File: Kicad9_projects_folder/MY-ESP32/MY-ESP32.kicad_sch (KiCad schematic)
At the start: 67 parts, among them J1 SM04B-SRSS-TB, J2 SM04B-SRSS-TB, Q1 2N3904S-RTK/PS, Q2 2N3904S-RTK/PS, Q5 PMOSFET-DMP1045U-7, SW3 SPDT, U1 USBLC6-2SC6, U3 CP2102N-Axx-xQFN28, U4 DFR0819, U7 USB4110GFA

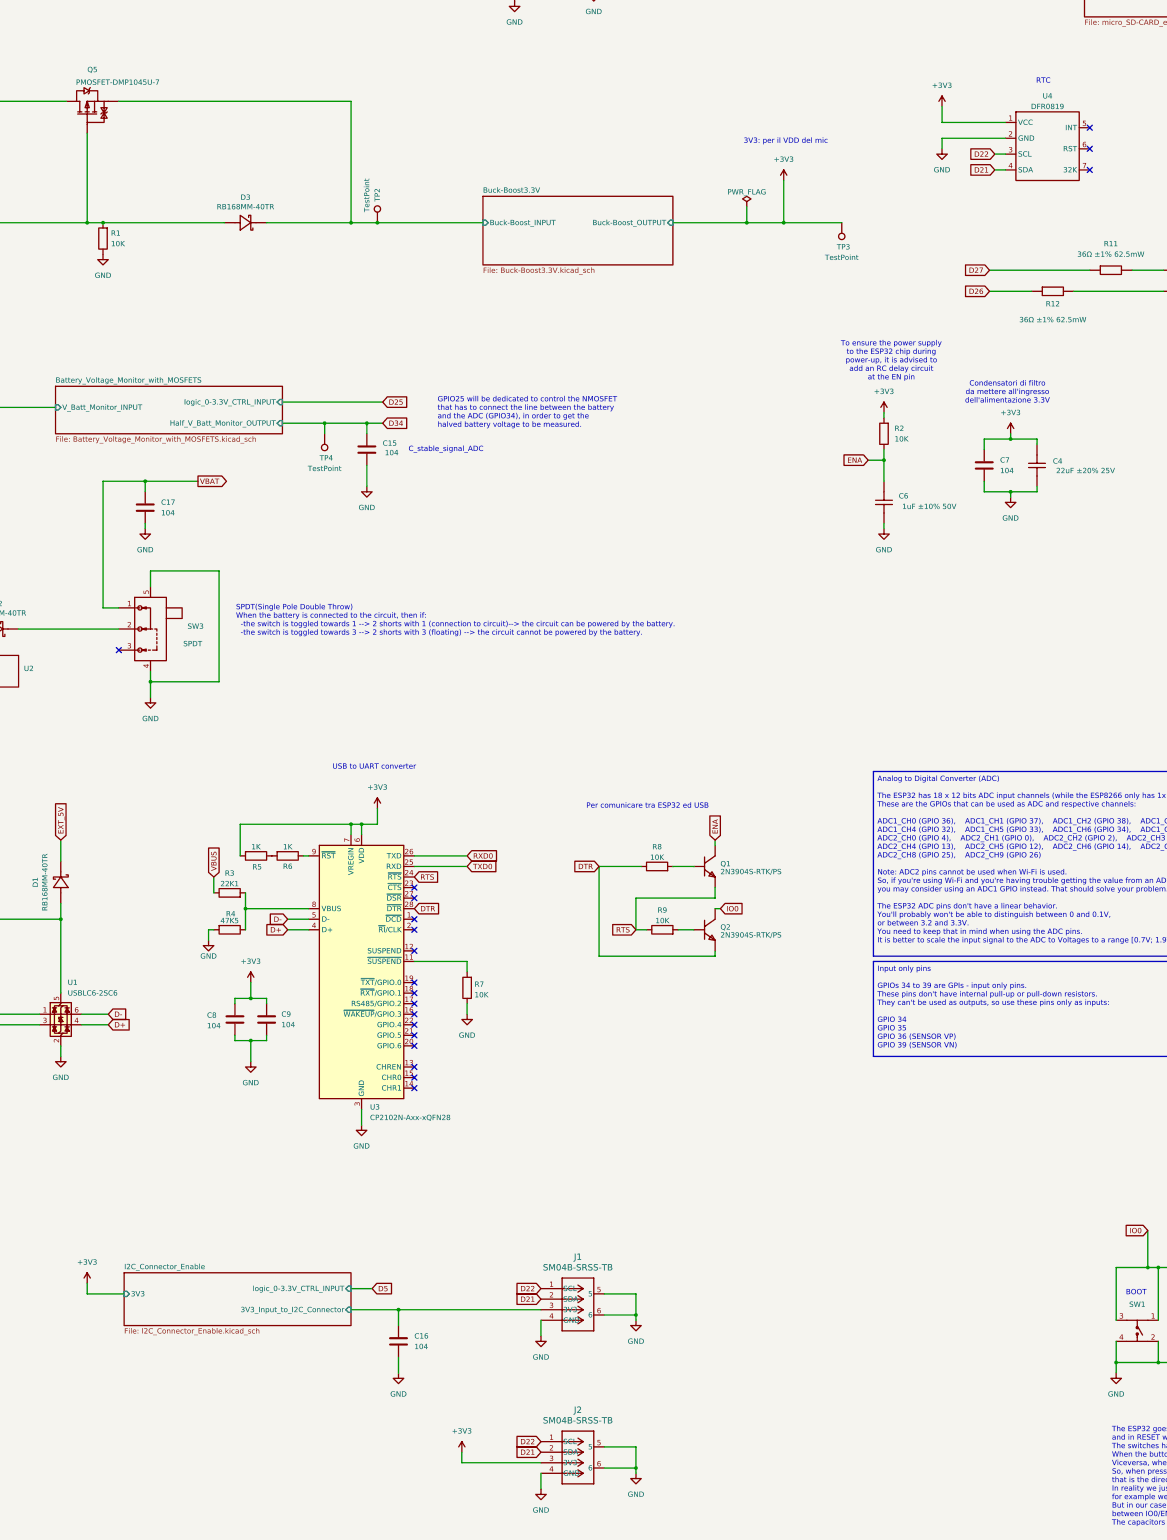
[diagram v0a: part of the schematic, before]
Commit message: Fourth commit
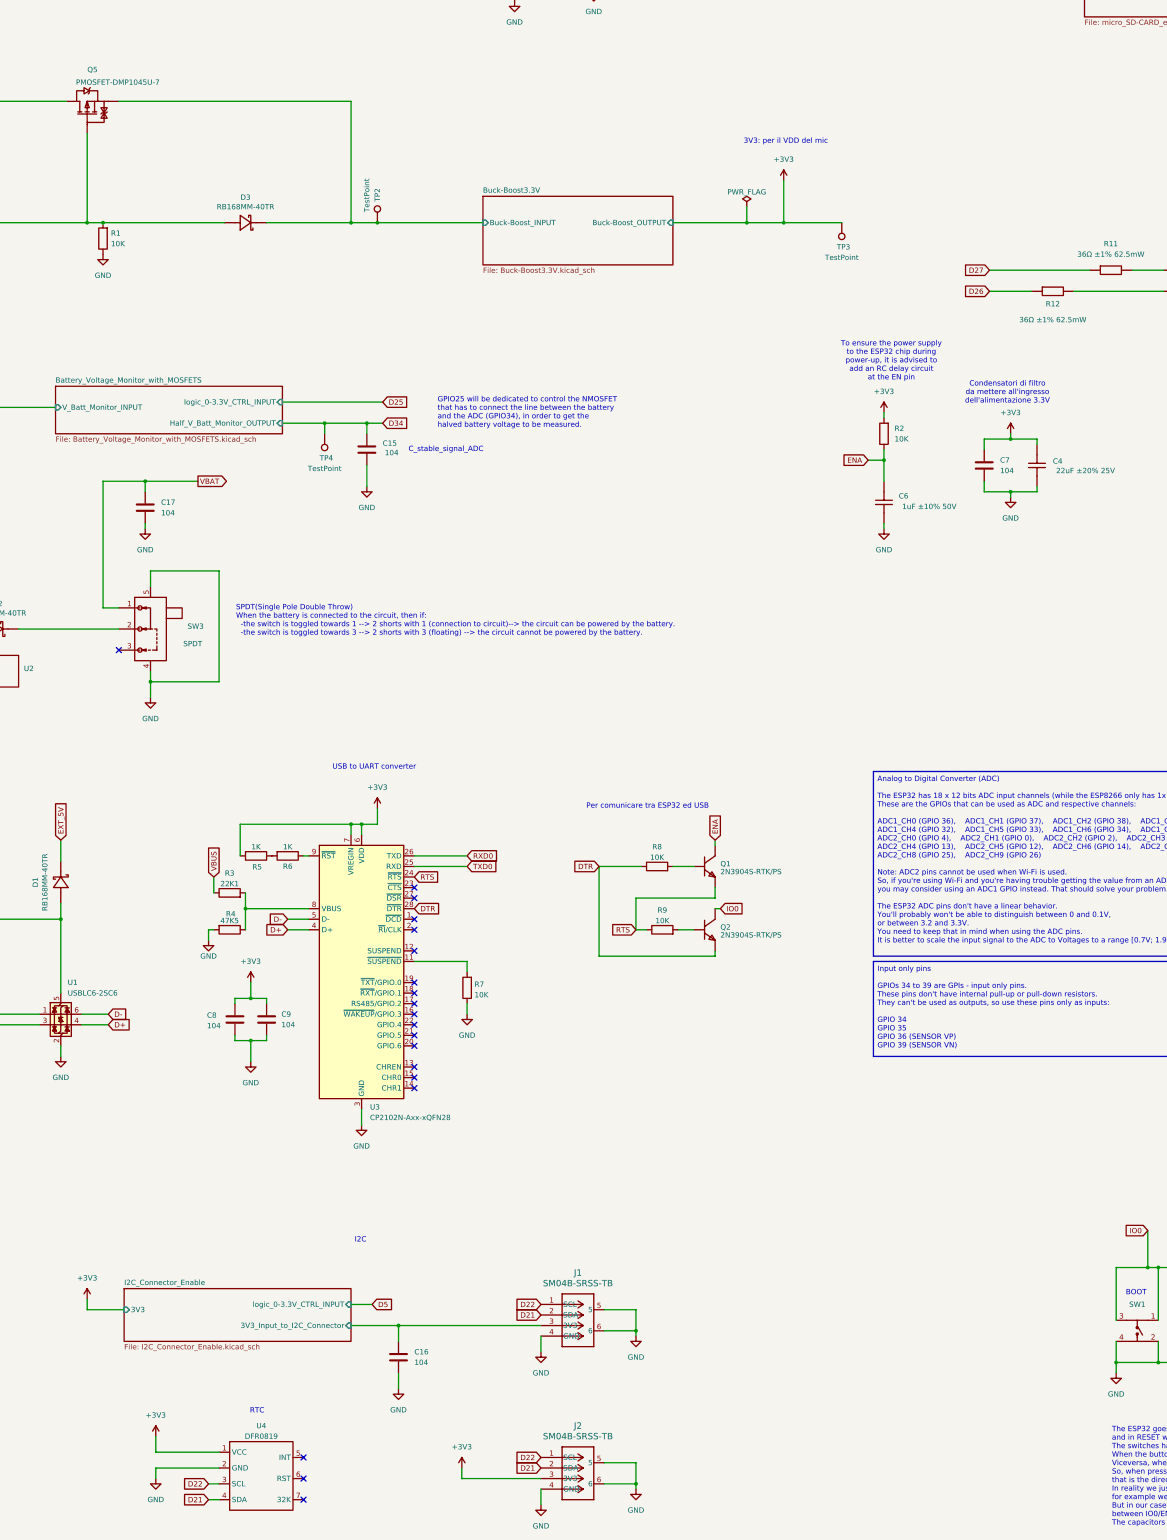
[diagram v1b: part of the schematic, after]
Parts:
- R10, R11, R12: footprint Resistor_SMD:R_0402_1005Metric -> My_Personal_Footprints_Library:RES_10K_0402WGF1002TCE
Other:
- note added: "I2C"
- moved on the sheet: C16, J1, J2, U4
